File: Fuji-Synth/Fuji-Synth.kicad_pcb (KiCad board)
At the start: 2 copper layers, 135.5 x 82.4 mm, 58 parts, among them J1 AudioJack3, SW1 RotaryEncoder_Switch, SW2 RotaryEncoder_Switch, SW3 SW_Push, SW4 RotaryEncoder_Switch, SW5 SW_Push, U1 PCM5102A, U2 ER_OLEDM0.91_1x-I2C, U3 MPR121QR2

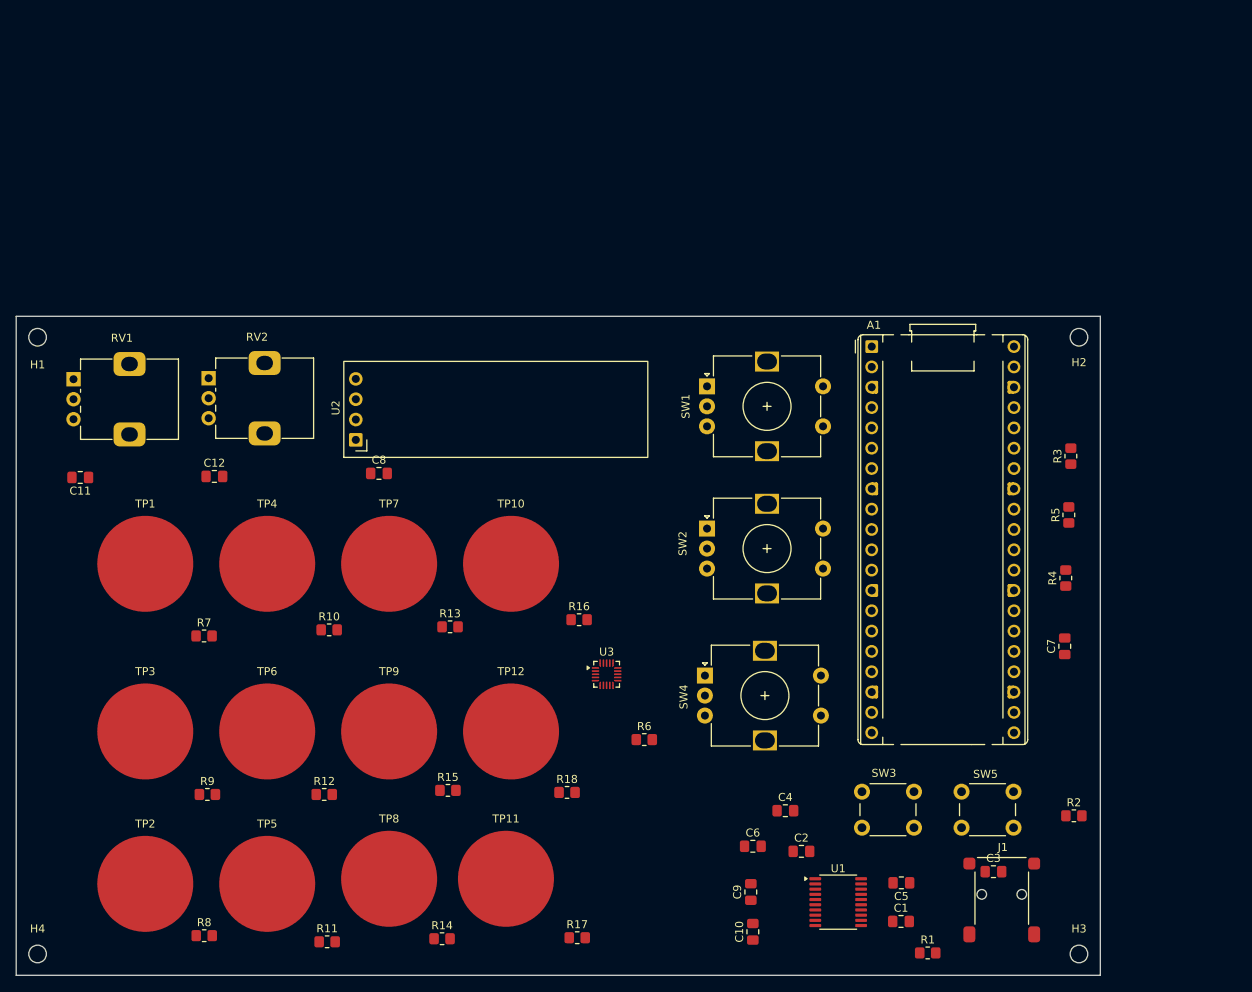
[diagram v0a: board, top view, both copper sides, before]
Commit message: PCB version 2 / removed old gerber files
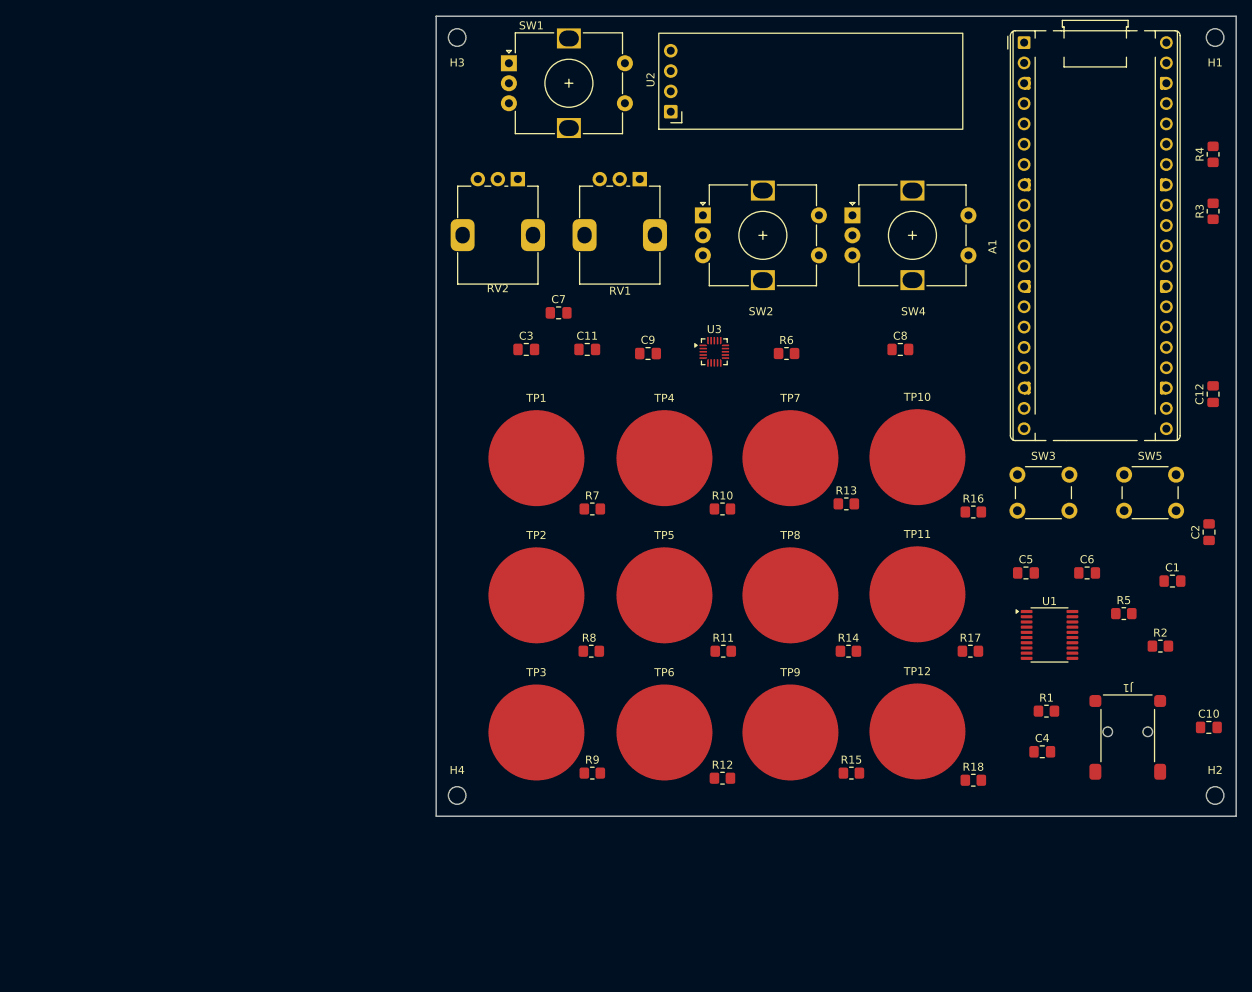
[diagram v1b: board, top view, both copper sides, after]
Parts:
- moved H1 151.9 mm to (169.9, 55.5), turned to 180 degrees
- moved H3 138.4 mm to (75.2, 55.5), turned to 180 degrees
- moved C12 125.3 mm to (169.7, 100.1), turned to 90 degrees
- moved C3 87.6 mm to (83.8, 94.5)
- moved C7 75.8 mm to (87.9, 89.9), turned to 0 degrees
- moved RV1 75.1 mm to (98.0, 73.2), turned to -90 degrees
- moved C9 68.5 mm to (99.0, 95.0), turned to 0 degrees
- moved C8 67.0 mm to (130.6, 94.5)
- moved C11 65.4 mm to (91.4, 94.5), turned to 0 degrees
- moved C2 64.7 mm to (169.2, 117.3), turned to 90 degrees
- moved TP11 62.5 mm to (132.7, 125.1)
- moved C10 62.5 mm to (169.1, 141.7), turned to 0 degrees
- moved R14 62.2 mm to (124.1, 132.2)
- moved TP8 61.4 mm to (116.8, 125.2)
- moved R11 61.4 mm to (108.4, 132.2)
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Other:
- board size 135.5 x 82.4 mm -> 100 x 100 mm
